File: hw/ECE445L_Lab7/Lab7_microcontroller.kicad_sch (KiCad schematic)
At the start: 21 parts, among them Y1 16MHz, Y2 16MHz

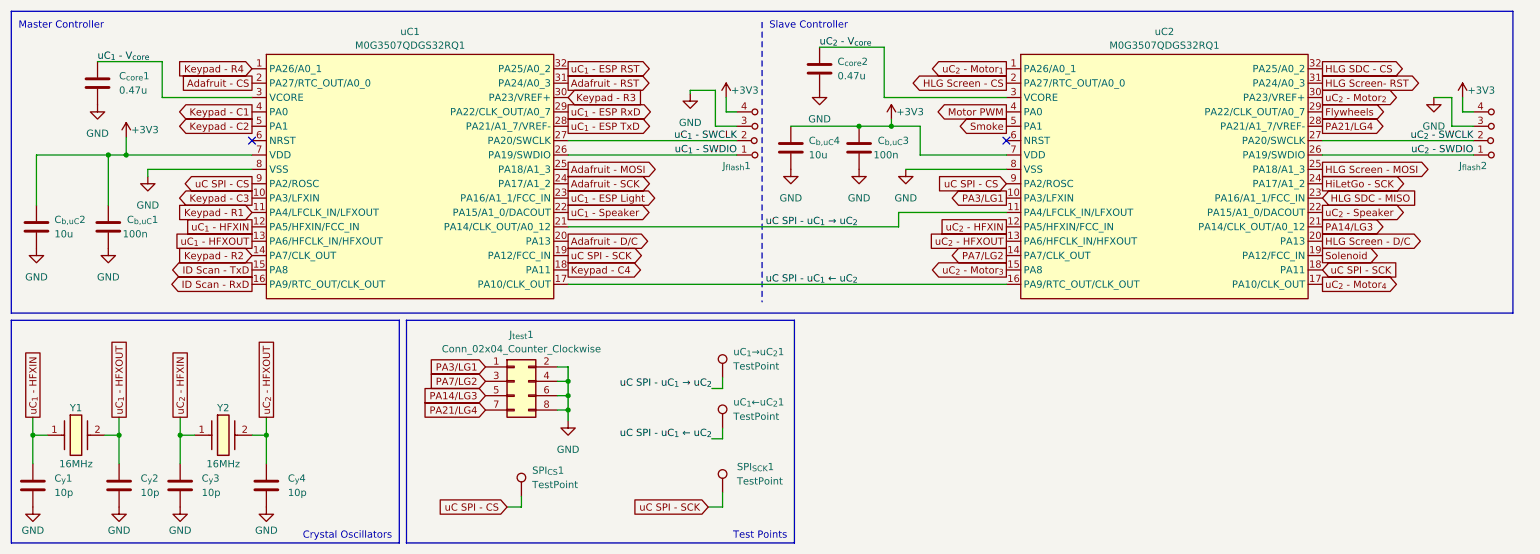
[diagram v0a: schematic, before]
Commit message: finished prelim layout for TA review
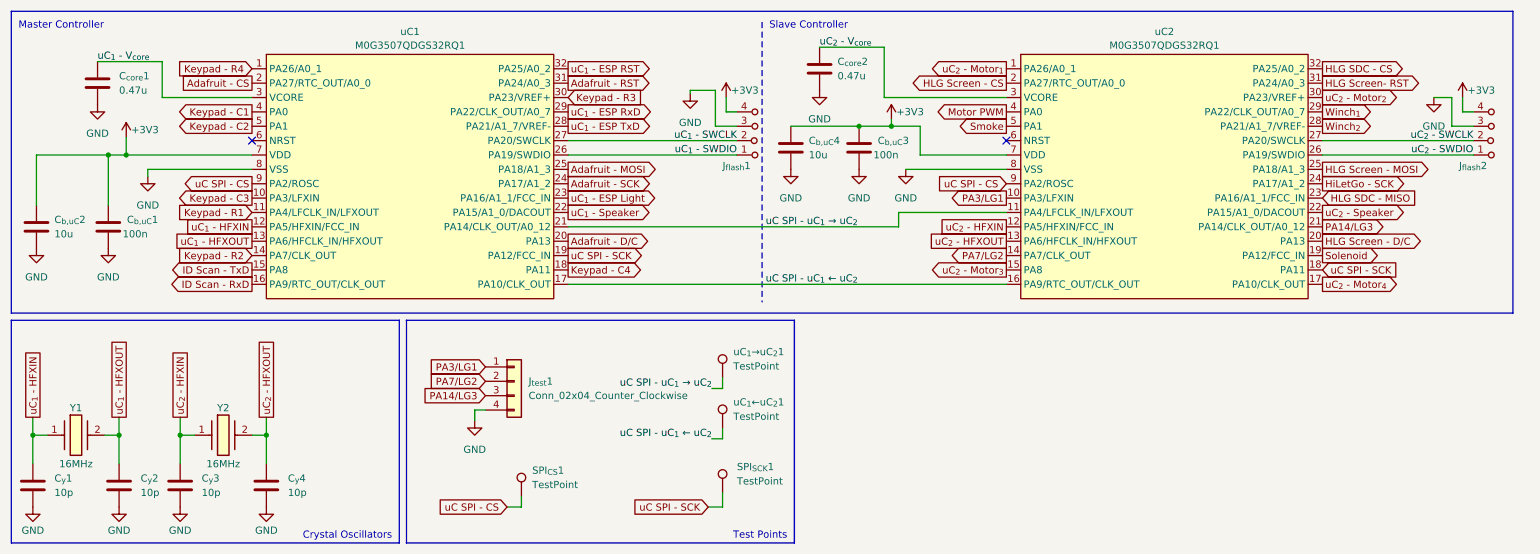
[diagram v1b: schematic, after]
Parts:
- J_{test}1: footprint Connector_PinSocket_2.54mm:PinSocket_2x04_P2.54mm_Vertical -> Connector_PinSocket_2.54mm:PinSocket_1x04_P2.54mm_Vertical; symbol Connector_Generic:Conn_02x04_Odd_Even -> Connector_Generic:Conn_01x04
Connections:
- net GND: no longer J_{test}1.2 (Pin_2), J_{test}1.6 (Pin_6), J_{test}1.8 (Pin_8)
- net PA14/LG3: now also J_{test}1.3 (Pin_3); no longer J_{test}1.5 (Pin_5)
- net PA7/LG2: now also J_{test}1.2 (Pin_2); no longer J_{test}1.3 (Pin_3)
- net Flywheels renamed Winch_{1}
- net PA21/LG4 renamed Winch_{2}
- net Winch_{2}: no longer J_{test}1.7 (Pin_7)
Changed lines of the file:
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@@
 	)
 	(junction
-		(at 112.395 128.905)
-		(diameter 0)
-		(color 0 0 0 0)
-	)
-	(junction
-		(at 112.395 126.365)
-		(diameter 0)
-		(color 0 0 0 0)
-	)
-	(junction
 		(at 31.115 86.36)
 		(diameter 0)
@@
 	)
 	(junction
-		(at 112.395 131.445)
-		(diameter 0)
-		(color 0 0 0 0)
-	)
-	(junction
 		(at 33.02 135.89)
 		(diameter 0)
@@
 	(wire
 		(pts
-			(xy 110.49 131.445) (xy 112.395 131.445)
-		)
-		(stroke
-			(width 0)
-			(type default)
-		)
-	)
-	(wire
-		(pts
 			(xy 265.43 76.2) (xy 268.605 76.2)
 		)
@@
 	(wire
 		(pts
-			(xy 112.395 128.905) (xy 112.395 131.445)
-		)
-		(stroke
-			(width 0)
-			(type default)
-		)
-	)
-	(wire
-		(pts
 			(xy 40.64 76.2) (xy 56.515 76.2)
 		)
@@
 	(wire
 		(pts
-			(xy 112.395 126.365) (xy 112.395 128.905)
+			(xy 97.79 131.445) (xy 95.885 131.445)
 		)
 		(stroke
@@
 	(wire
 		(pts
-			(xy 110.49 126.365) (xy 112.395 126.365)
-		)
-		(stroke
-			(width 0)
-			(type default)
-		)
-	)
-	(wire
-		(pts
 			(xy 59.055 132.715) (xy 59.055 135.89)
 		)
@@
 	(wire
 		(pts
-			(xy 110.49 128.905) (xy 112.395 128.905)
-		)
-		(stroke
-			(width 0)
-			(type default)
-		)
-	)
-	(wire
-		(pts
-			(xy 112.395 123.825) (xy 112.395 126.365)
+			(xy 18.415 86.36) (xy 31.115 86.36)
 		)
 		(stroke
@@
 	(wire
 		(pts
-			(xy 18.415 86.36) (xy 31.115 86.36)
+			(xy 17.78 132.715) (xy 17.78 135.89)
 		)
 		(stroke
@@
 	(wire
 		(pts
-			(xy 17.78 132.715) (xy 17.78 135.89)
+			(xy 34.29 83.185) (xy 34.29 86.36)
 		)
 		(stroke
@@
 	(wire
 		(pts
-			(xy 34.29 83.185) (xy 34.29 86.36)
+			(xy 101.6 148.59) (xy 104.14 148.59)
 		)
 		(stroke
@@
 	(wire
 		(pts
-			(xy 101.6 148.59) (xy 104.14 148.59)
+			(xy 95.885 131.445) (xy 95.885 133.35)
 		)
 		(stroke
@@
 	(wire
 		(pts
-			(xy 112.395 131.445) (xy 112.395 133.35)
-		)
-		(stroke
-			(width 0)
-			(type default)
-		)
-	)
-	(wire
-		(pts
 			(xy 139.7 134.62) (xy 139.7 136.525)
 		)
@@
 	(wire
 		(pts
-			(xy 110.49 123.825) (xy 112.395 123.825)
-		)
-		(stroke
-			(width 0)
-			(type default)
-		)
-	)
-	(wire
-		(pts
 			(xy 43.815 140.97) (xy 43.815 135.89)
 		)
@@
 		)
 	)
-	(global_label "Flywheels"
+	(global_label "Winch_{1}"
 		(shape output)
 		(at 245.745 78.74 0)
@@
 		)
 		(property "Intersheetrefs" "${INTERSHEET_REFS}"
-			(at 264.6958 78.74 0)
+			(at 255.4817 78.74 0)
 			(hide yes)
 			(show_name no)
@@
 		)
 	)
-	(global_label "PA21{slash}LG4"
+	(global_label "Winch_{2}"
 		(shape output)
 		(at 245.745 81.28 0)
@@
 		)
 		(property "Intersheetrefs" "${INTERSHEET_REFS}"
-			(at 258.3459 81.28 0)
+			(at 255.4817 81.28 0)
 			(hide yes)
 			(show_name no)
@@
 		)
 	)
-	(global_label "PA21{slash}LG4"
-		(shape input)
-		(at 97.79 131.445 180)
-		(fields_autoplaced yes)
-		(effects
-			(font
-				(size 1.27 1.27)
-			)
-			(justify right)
-		)
-		(property "Intersheetrefs" "${INTERSHEET_REFS}"
-			(at 85.1891 131.445 0)
-			(hide yes)
-			(show_name no)
-			(do_not_autoplace no)
-			(effects
-				(font
-					(size 1.27 1.27)
-				)
-				(justify right)
-			)
-		)
-	)
 	(global_label "ID Scan - RxD"
 		(shape output)
@@
 		)
 	)
+	(rule_area
+		(exclude_from_sim no)
+		(in_bom yes)
+		(on_board yes)
+		(dnp no)
+		(polyline
+			(pts
+				(xy 14.605 116.205) (xy 67.31 116.205) (xy 67.31 154.305) (xy 14.605 154.305)
+			)
+			(stroke
+				(width 0)
+				(type dash)
+			)
+			(fill
+				(type none)
+			)
+		)
+	)
+	(netclass_flag ""
+		(length 2.54)
+		(shape round)
+		(at 67.31 128.905 270)
+		(fields_autoplaced yes)
+		(effects
+			(font
+				(size 1.27 1.27)
+			)
+			(justify right bottom)
+		)
+		(property "Netclass" "CrystalTrace"
+			(at 69.85 128.2065 90)
+			(show_name no)
+			(do_not_autoplace no)
+			(effects
+				(font
+					(size 1.27 1.27)
+				)
+				(justify left)
+			)
+		)
+		(property "Component Class" ""
+			(at -53.34 17.145 0)
+			(show_name no)
+			(do_not_autoplace no)
+			(effects
+				(font
+					(size 1.27 1.27)
+					(italic yes)
+				)
+			)
+		)
+	)
 	(symbol
 		(lib_id "ECE445L:ABM3-16.000MHZ-B2-T")
@@
 	(symbol
 		(lib_id "power:GND")
-		(at 112.395 133.35 0)
+		(at 95.885 133.35 0)
 		(unit 1)
 		(body_style 1)
@@
 		(fields_autoplaced yes)
 		(property "Reference" "#PWR041"
-			(at 112.395 139.7 0)
+			(at 95.885 139.7 0)
 			(hide yes)
 			(show_name no)
@@
 		)
 		(property "Value" "GND"
-			(at 112.395 138.43 0)
+			(at 95.885 138.43 0)
 			(show_name no)
 			(do_not_autoplace no)
@@
 		)
 		(property "Footprint" ""
-			(at 112.395 133.35 0)
+			(at 95.885 133.35 0)
 			(hide yes)
 			(show_name no)
@@
 		)
 		(property "Datasheet" ""
-			(at 112.395 133.35 0)
+			(at 95.885 133.35 0)
 			(hide yes)
 			(show_name no)
@@
 		)
 		(property "Description" "Power symbol creates a global label with name \"GND\" , ground"
-			(at 112.395 133.35 0)
+			(at 95.885 133.35 0)
 			(hide yes)
 			(show_name no)
@@
 	)
 	(symbol
-		(lib_id "Connector_Generic:Conn_02x04_Odd_Even")
+		(lib_id "Connector_Generic:Conn_01x04")
 		(at 102.87 126.365 0)
 		(unit 1)
@@
 		(fields_autoplaced yes)
 		(property "Reference" "J_{test}1"
-			(at 104.14 118.11 0)
+			(at 105.41 126.3649 0)
 			(show_name no)
 			(do_not_autoplace no)
@@
 					(size 1.27 1.27)
 				)
+				(justify left)
 			)
 		)
 		(property "Value" "Conn_02x04_Counter_Clockwise"
-			(at 104.14 120.65 0)
+			(at 105.41 128.9049 0)
 			(show_name no)
 			(do_not_autoplace no)
@@
 					(size 1.27 1.27)
 				)
+				(justify left)
 			)
 		)
-		(property "Footprint" "Connector_PinSocket_2.54mm:PinSocket_2x04_P2.54mm_Vertical"
+		(property "Footprint" "Connector_PinSocket_2.54mm:PinSocket_1x04_P2.54mm_Vertical"
 			(at 102.87 126.365 0)
 			(hide yes)
@@
 			)
 		)
-		(property "Description" "Generic connector, double row, 02x04, odd/even pin numbering scheme (row 1 odd numbers, row 2 even numbers), script generated (kicad-library-utils/schlib/autogen/connector/)"
+		(property "Description" "Generic connector, single row, 01x04, script generated (kicad-library-utils/schlib/autogen/connector/)"
 			(at 102.87 126.365 0)
 			(hide yes)
@@
 			)
 		)
-		(pin "6"
-		)
-		(pin "5"
-		)
 		(pin "3"
 		)
-		(pin "8"
-		)
 		(pin "4"
 		)
@@
 		(pin "2"
 		)
-		(pin "7"
-		)
 		(instances
